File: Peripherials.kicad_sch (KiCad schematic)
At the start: 25 parts, among them J13 USB_C_Receptacle_USB2.0_14P, J14 IDC_Cable_02x08, J15 Conn_01x02_Pin, J18 Micro_SD_Card, Q2 NMOS, U13 USBLC6-2P6, U2 RV-3028-C7

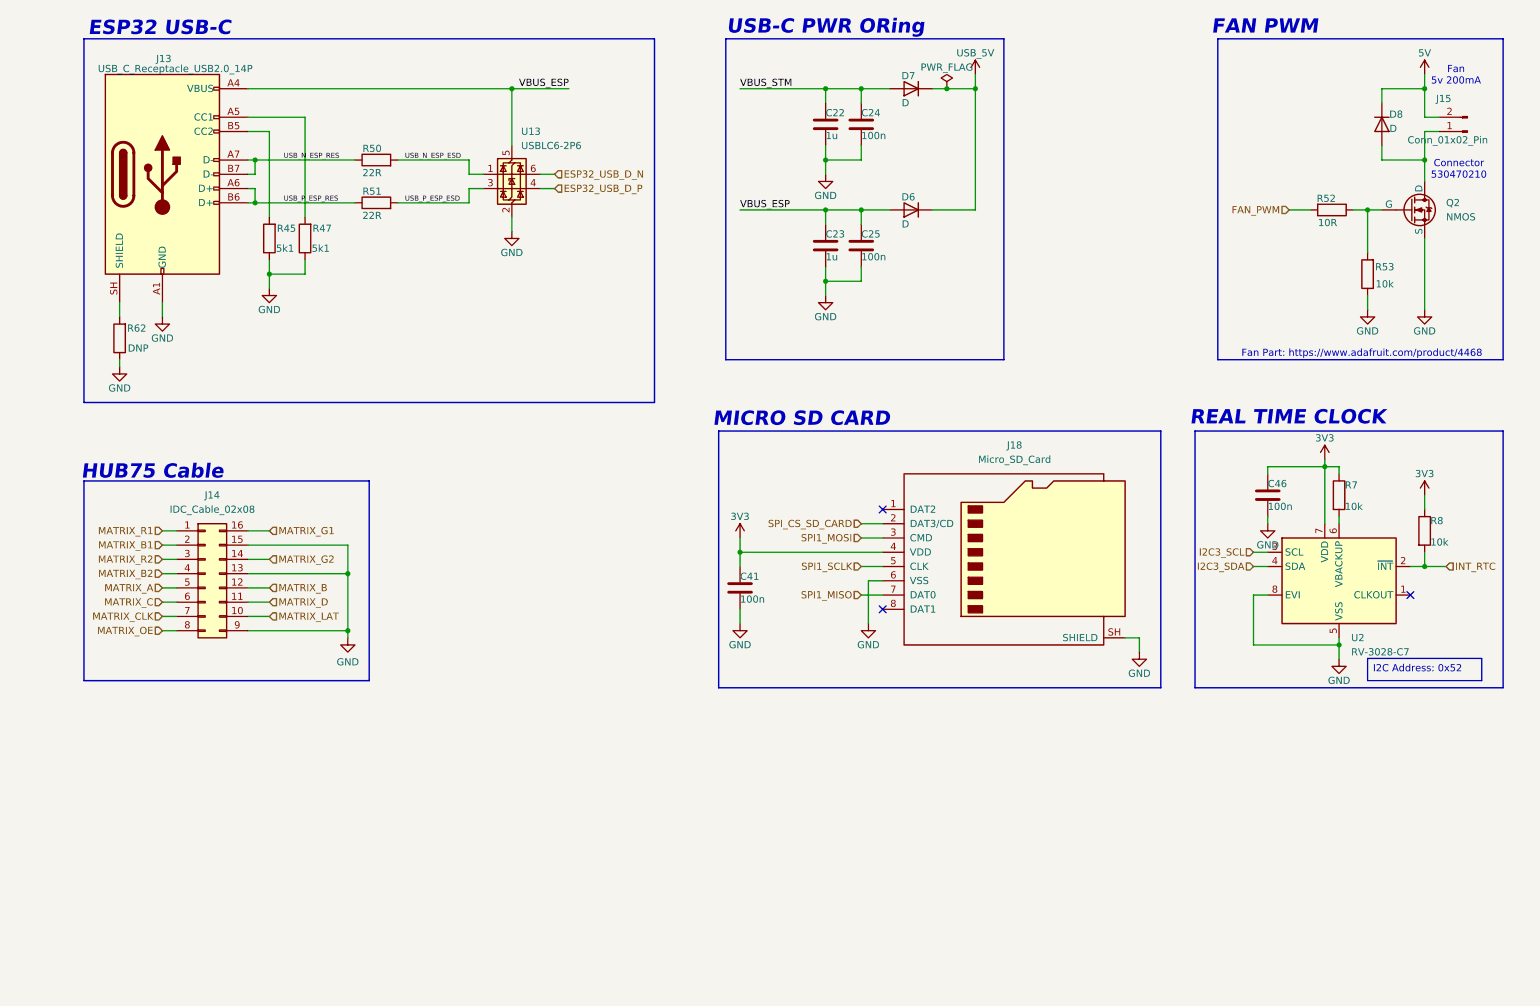
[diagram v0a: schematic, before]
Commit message: fixing xander's push
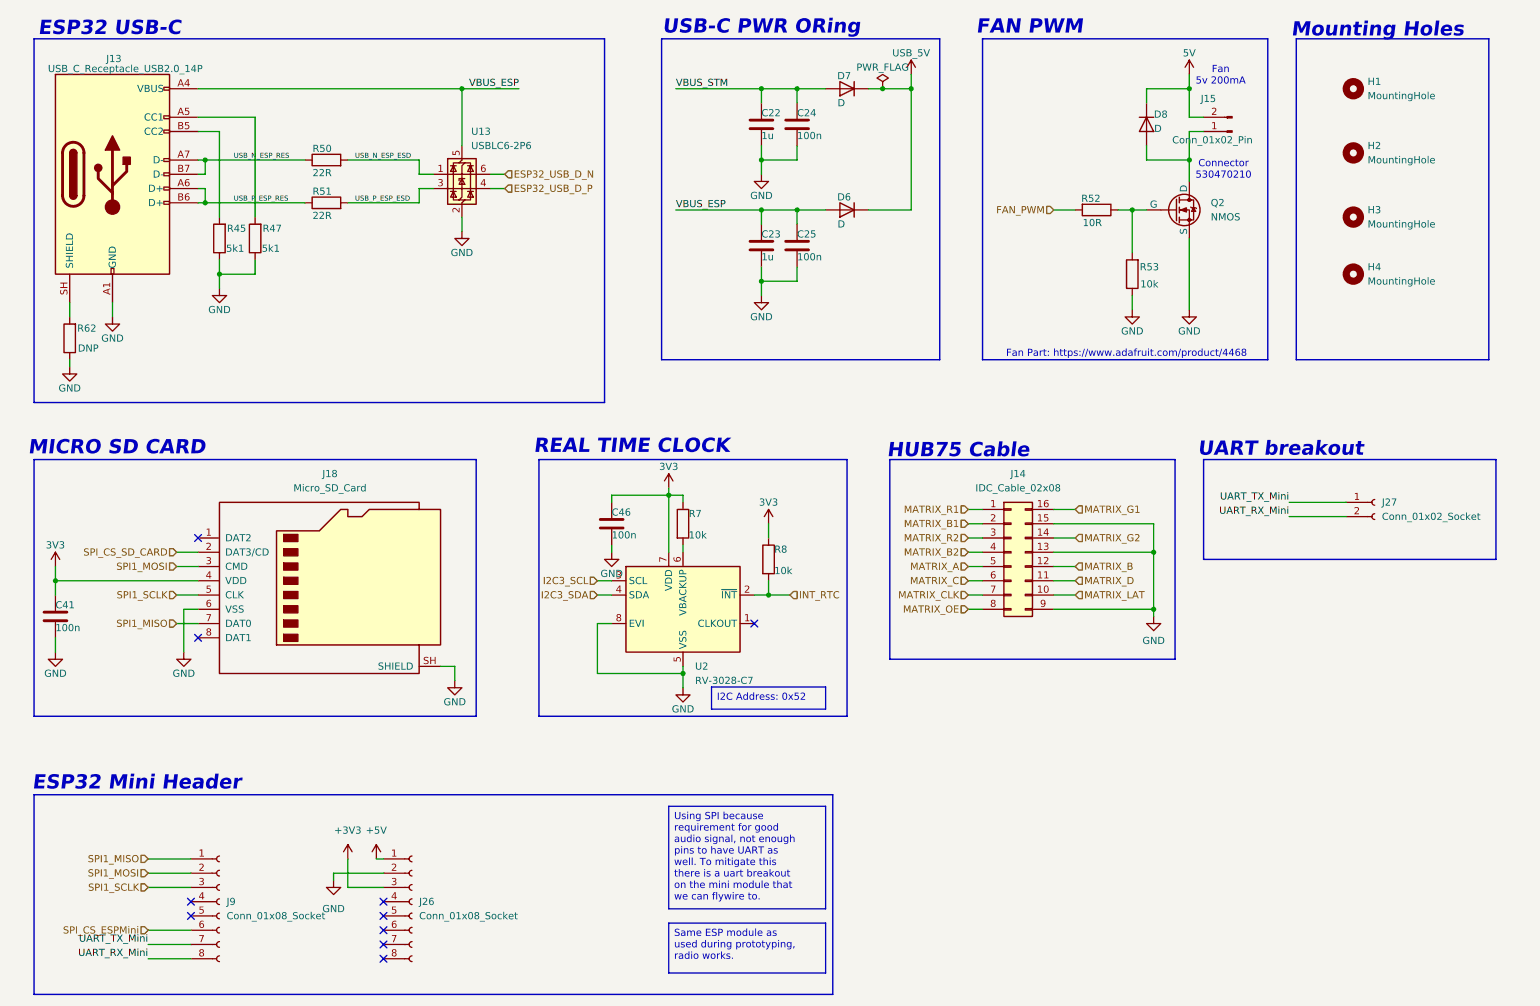
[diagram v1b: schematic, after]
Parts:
- added H1, H2, H3, H4: MountingHole, MountingHole:MountingHole_3.2mm_M3, symbol Mechanical:MountingHole
- added J26, J9: Conn_01x08_Socket, Connector_PinHeader_2.54mm:PinHeader_1x08_P2.54mm_Vertical, symbol Connector:Conn_01x08_Socket
- added J27: Conn_01x02_Socket, Connector_PinHeader_2.54mm:PinHeader_1x02_P2.54mm_Vertical, symbol Connector:Conn_01x02_Socket
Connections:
- net GND: now also J26.2 (Pin_2)
- net SPI1_MISO: now also J9.1 (Pin_1)
- net SPI1_MOSI: now also J9.2 (Pin_2)
- net SPI1_SCLK: now also J9.3 (Pin_3)
- new net +3V3: J26.3 (Pin_3)
- new net +5V: J26.1 (Pin_1)
- new net SPI_CS_ESPMini: J9.6 (Pin_6)
- new net UART_RX_Mini: J27.2 (Pin_2), J9.8 (Pin_8)
- new net UART_TX_Mini: J27.1 (Pin_1), J9.7 (Pin_7)
- no-connect marks 3 -> 10
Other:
- note added: "ESP32 Mini Header"
- note added: "Mounting Holes"
- note added: "UART breakout"
